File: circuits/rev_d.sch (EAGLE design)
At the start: 16 parts, among them X1 ENCODER_ANO

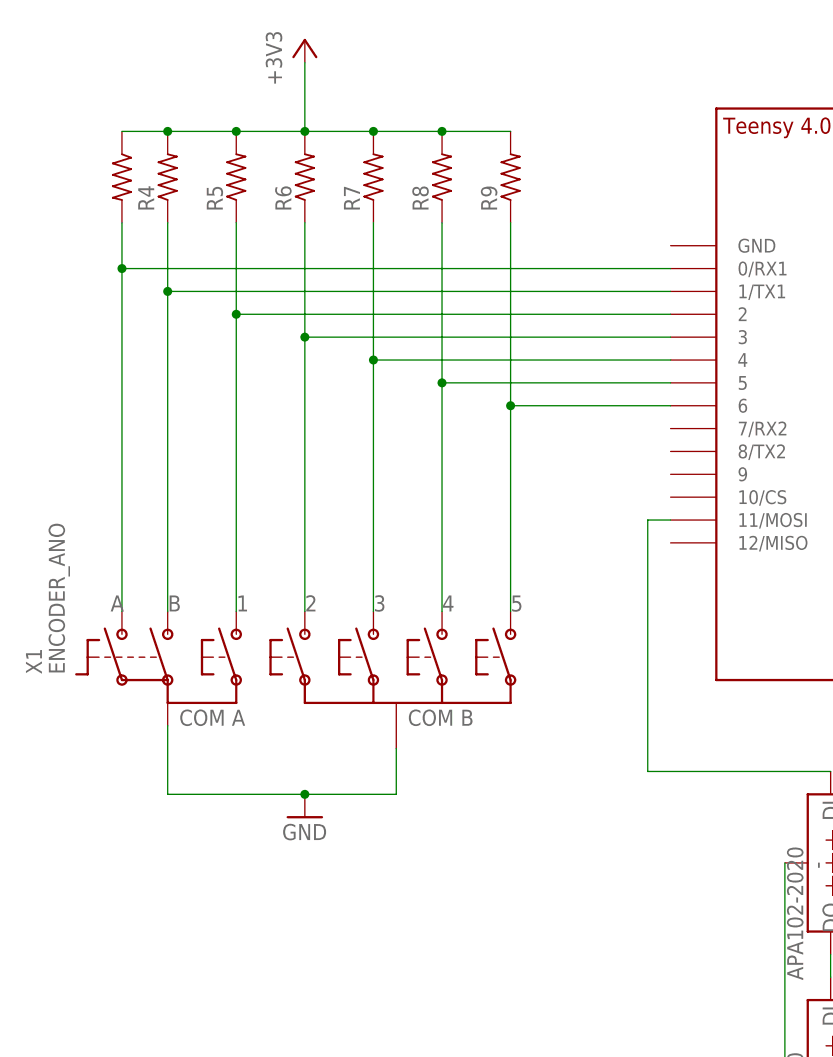
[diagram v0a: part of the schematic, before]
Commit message: Working through feature suggestions.
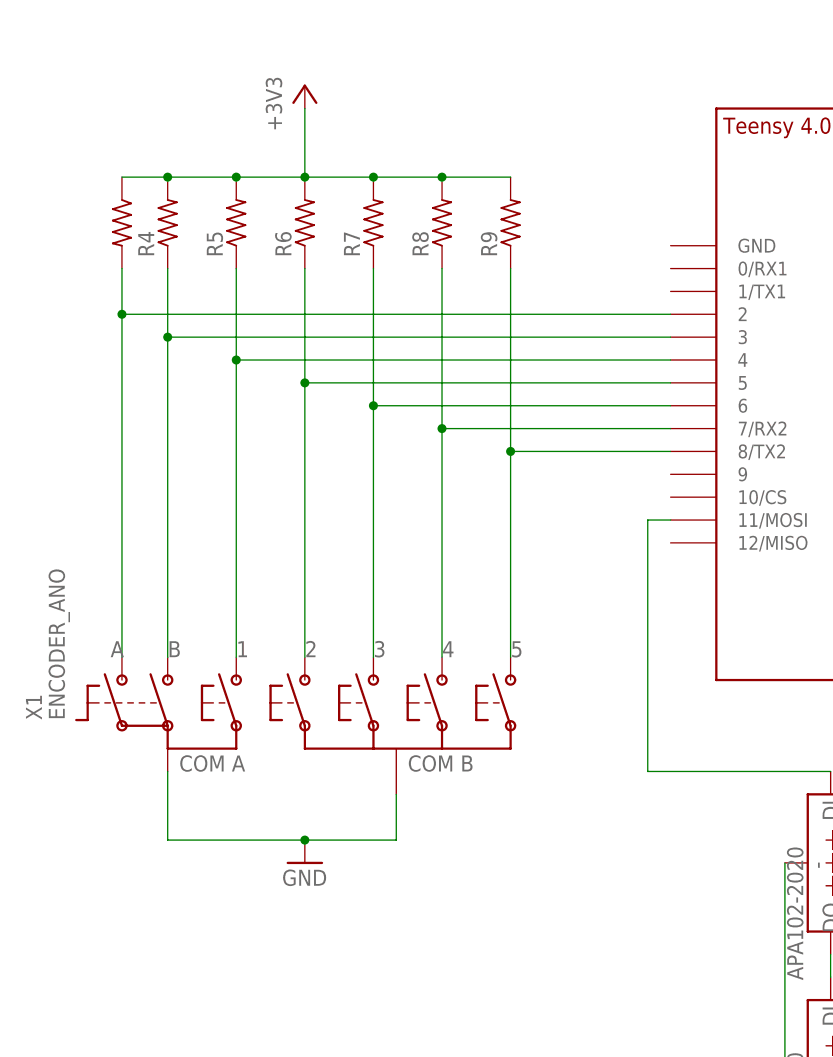
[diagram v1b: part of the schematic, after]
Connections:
- net N$1: now also MCU.8/TX2; no longer MCU.6
- net N$2: now also MCU.7/RX2; no longer MCU.5
- net N$3: now also MCU.6; no longer MCU.4
- net N$4: now also MCU.5; no longer MCU.3
- net N$5: now also MCU.4; no longer MCU.2
- net N$6: now also MCU.3; no longer MCU.1/TX1
- net N$7: now also MCU.2; no longer MCU.0/RX1
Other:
- moved on the sheet: R4, R5, R6, R7, R8, R9, X1
